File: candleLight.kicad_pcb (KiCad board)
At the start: 2 copper layers, 38.8 x 20 mm, 43 parts, among them P1 USB_C_Plug_USB2.0, U201 STM32F072C8Tx, U301 MCP1754ST-3302E/MB, U401 TJA1051/3, X501 CON_SWD, X502 SUB-D9, Y201 8MHz

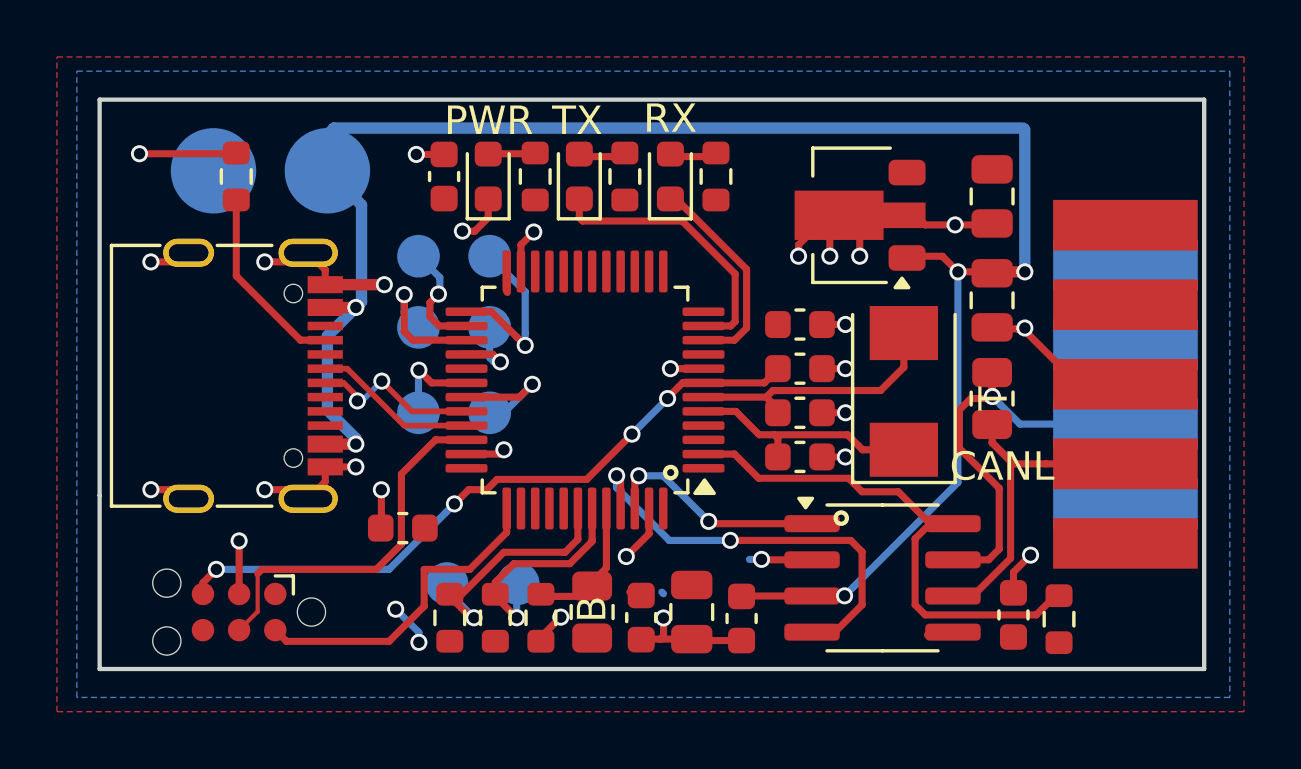
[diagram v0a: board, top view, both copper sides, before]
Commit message: schematic
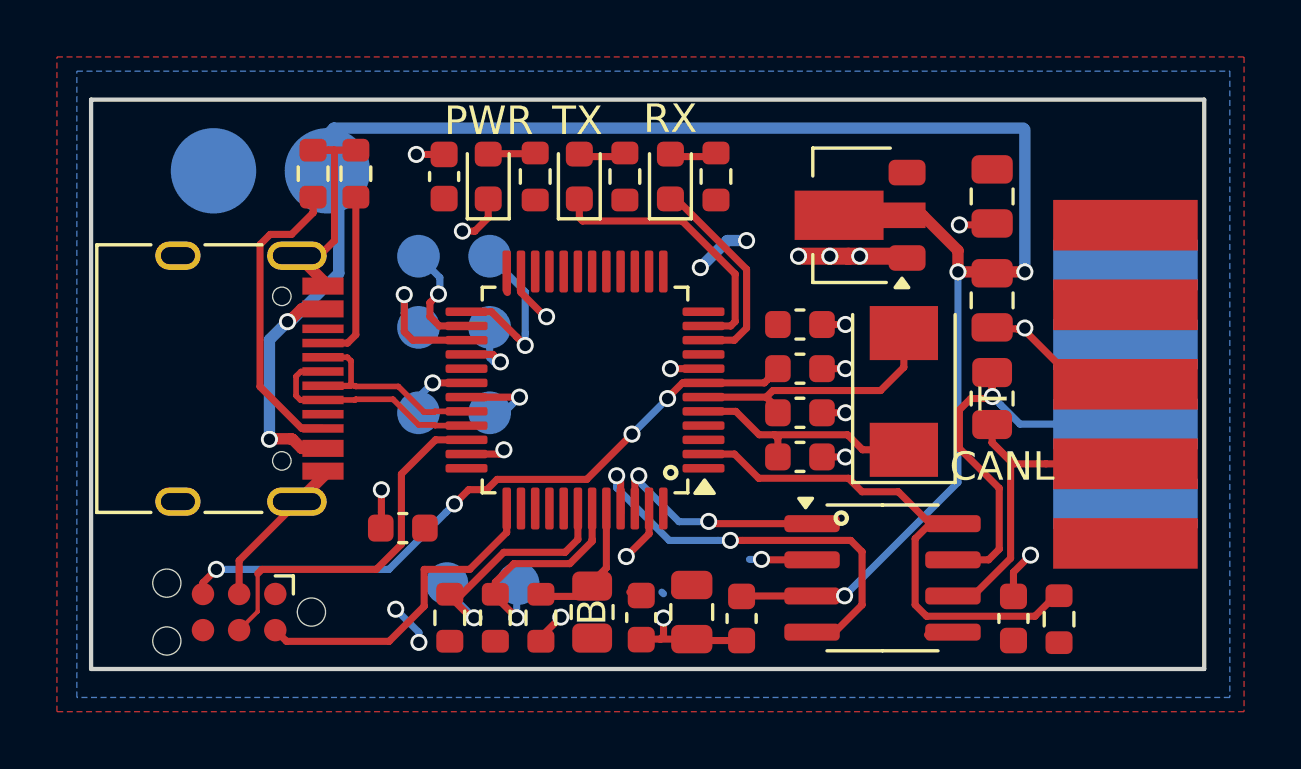
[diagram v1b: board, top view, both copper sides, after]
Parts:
- removed P1: USB_C_Plug_USB2.0, Connector_USB:USB_C_Receptacle_G-Switch_GT-USB-7010ASV
- removed the R1 at (45.1, 77.7)
- added J1: USB_C_Receptacle_USB2.0, stm32world:USB_C_Receptacle_HRO_TYPE-C-31-M-12, F.Cu at (44.1, 84.8)
- added R11: 5k1, Resistor_SMD:R_0603_1608Metric, F.Cu at (47.8, 77.6)
- added R5: 5k1, Resistor_SMD:R_0603_1608Metric, F.Cu at (49.3, 77.6)
- SCL1: renamed from W203; value TEST_1P -> SCL1
- SDA1: renamed from W204; value TEST_1P -> SDA1
- U1: renamed from U301; value MCP1754ST-3302E/MB -> ME6210A33PG
- moved G*** 1.20 mm to (64.1, 84.9)
- moved C12 0.12 mm to (72.4, 93.2)
- renumbered C301 to C1, C207 to C10, C402 to C11, C403 to C12, C303 to C2, C201 to C3, C202 to C4, C208 to C5, C203 to C6, C204 to C7, C205 to C8, C206 to C9, D601 to D1, D602 to D2, D603 to D3, R201 to R1, R603 to R10, R202 to R2, R203 to R3, R204 to R4, R401 to R6, R402 to R7, R601 to R8, R602 to R9, U201 to U2, U401 to U3, W301 to W1, W302 to W2, W205 to W3, W206 to W4, W207 to W5, W208 to W6, W201 to W7, W202 to W8, X501 to X1, X502 to X2, Y201 to Y1
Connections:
- net /CAN/CAN_H renamed CAN_H
- net /CAN/CAN_L renamed CAN_L
- net /CAN/CAN_RXD renamed CAN_RX
- net /CAN/CAN_S renamed /CAN_S
- net /CAN/CAN_TXD renamed CAN_TX
- net /Connectors/NRST renamed NRST
- net /Connectors/SWCLK renamed SWCLK
- net /Connectors/SWDIO renamed SWDIO
- net /LEDs/LED1 renamed LED1
- net /LEDs/LED2 renamed LED2
- net /MCU/BOOT0 renamed Net-(U2-BOOT0)
- U1 pad 1: +5V -> GND
- U1 pad 2: GND -> +5V
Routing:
- net Net-(J1-CC2): track 0.00 -> 10.7 mm
- net GND: track 54.9 -> 47.9 mm, vias 28 -> 20
- net Net-(P1-CC): track 6.73 -> 0.00 mm
- net Net-(J1-CC1): track 0.00 -> 5.97 mm
- net +5V: track 64.9 -> 67.4 mm
- net USB_DP: track 5.79 -> 8.18 mm
- net USB_DN: track 6.16 -> 8.20 mm, vias 2 -> 0
- net +3V3: track 5.57 -> 7.59 mm, vias 2 -> 4
- net Net-(U2-PA10): track 4.60 -> 3.33 mm
- net Net-(U2-PA9): track 3.17 -> 2.44 mm
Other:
- board size 38.8 x 20 mm -> 39.1 x 20 mm
